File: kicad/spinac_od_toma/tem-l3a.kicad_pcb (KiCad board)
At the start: 2 copper layers, 14 parts, among them J1 Conn_01x02_Male, SW1 SW_Push, SW2 SW_Push, U1 LM555xM

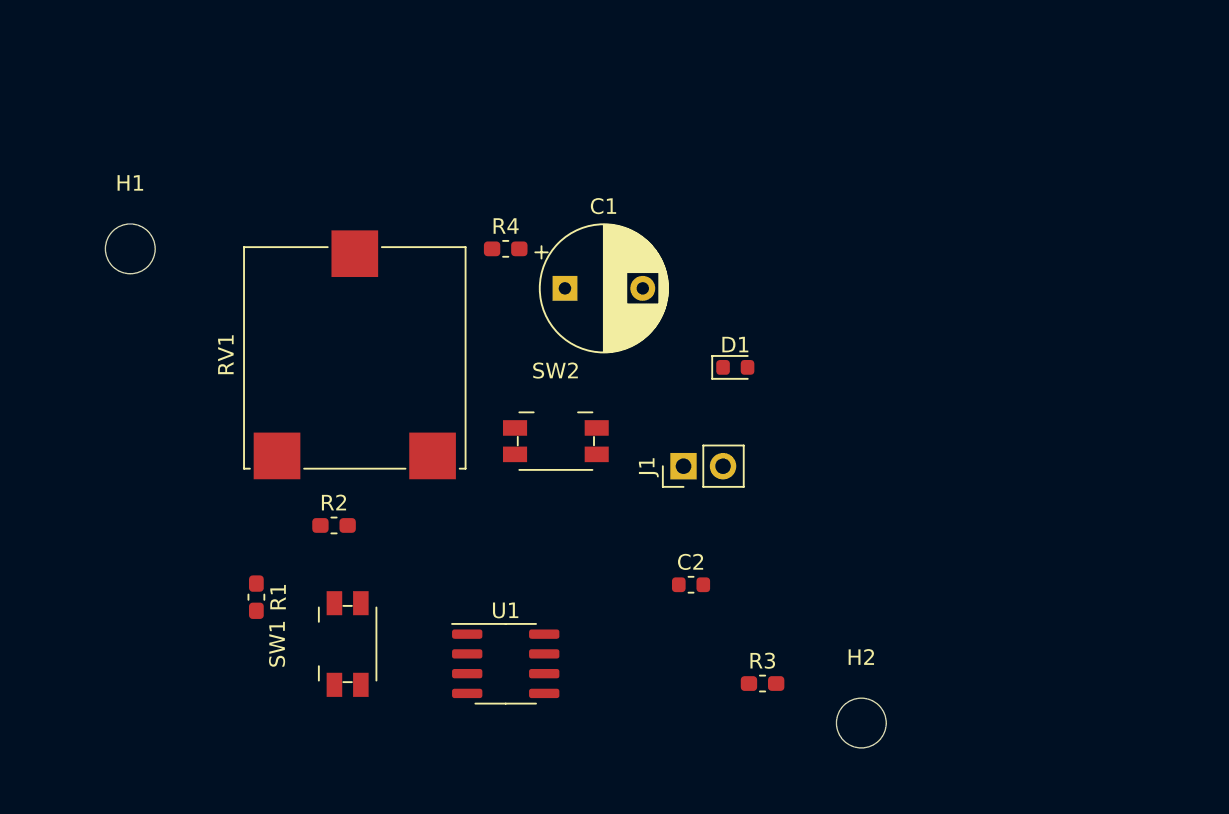
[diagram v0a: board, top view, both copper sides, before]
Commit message: t
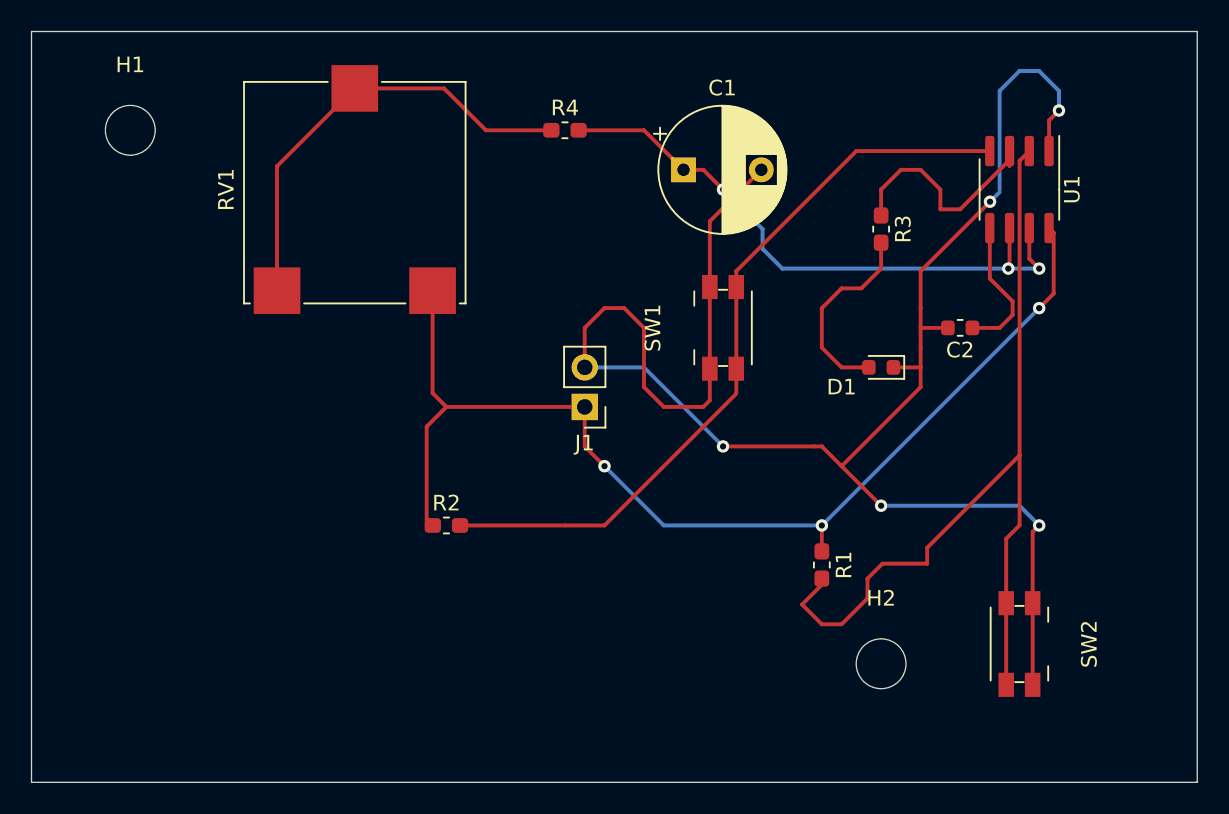
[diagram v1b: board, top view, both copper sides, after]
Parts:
- moved U1 44.9 mm to (189.2, 87.6), turned to 270 degrees
- moved R1 36.4 mm to (176.5, 111.8)
- moved SW2 32.5 mm to (189.2, 116.8), turned to 270 degrees
- moved SW1 31.5 mm to (170.2, 96.5)
- moved R3 30.2 mm to (180.3, 90.2), turned to 270 degrees
- moved C2 23.9 mm to (185.4, 96.5), turned to 180 degrees
- moved C1 10.8 mm to (167.6, 86.4)
- moved RV1 10.6 mm to (146.5, 87.6)
- moved D1 9.37 mm to (180.3, 99.1), turned to 180 degrees
- moved R4 8.52 mm to (160.0, 83.8)
- moved H1 7.62 mm to (132.1, 83.8)
- moved J1 7.41 mm to (161.3, 101.6), turned to 180 degrees
- moved R2 7.22 mm to (152.4, 109.2)
- moved H2 4.02 mm to (180.3, 118.1)
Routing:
- net Net-(C1-Pad2): track 0.00 -> 118.1 mm, vias 0 -> 5
- net Net-(J1-Pad1): track 0.00 -> 72.0 mm, vias 0 -> 3
- net Net-(R1-Pad2): track 0.00 -> 57.5 mm
- net Net-(R2-Pad2): track 0.00 -> 48.6 mm
- net Net-(C1-Pad1): track 0.00 -> 39.5 mm, vias 0 -> 3
- net Net-(R4-Pad1): track 0.00 -> 28.8 mm
- net Net-(R3-Pad1): track 0.00 -> 15.1 mm
- net Net-(D1-Pad2): track 0.00 -> 13.1 mm
- net Net-(C2-Pad1): track 0.00 -> 9.12 mm
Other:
- board outline added: 74.9 x 48.3 mm

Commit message: lul
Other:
- net class Default removed
